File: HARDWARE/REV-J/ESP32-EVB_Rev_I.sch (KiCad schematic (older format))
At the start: 151 parts, among them CON1 TB3 DG306-5.0-3P, CON2 TB3 DG306-5.0-3P, Q1 BC817-40(SOT23), Q2 BC817-40(SOT23), Q3 Q12MHz/20pF/30ppm/2P/HC-49SM(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, Q4 BC817-40(SOT23), Q5 BC817-40(SOT23), Q7 BC817-40(SOT23), U1 BL4054B-42TPRN(SOT23-5), U10 BAT54C(SOT23-3), U2 SY8089AAAC(SOT23-5), U3 ESP-WROOM-32, U4 LAN8710A-EZC(QFN32), U5 CH340T(SSOP20W), U6 MCP2562-E/SN(SOIC-8_150mil), U7 RPM7236-H8, U8 NCP303LSN27T1G(SOT-23-5), U9 BAT54C(SOT23-3)

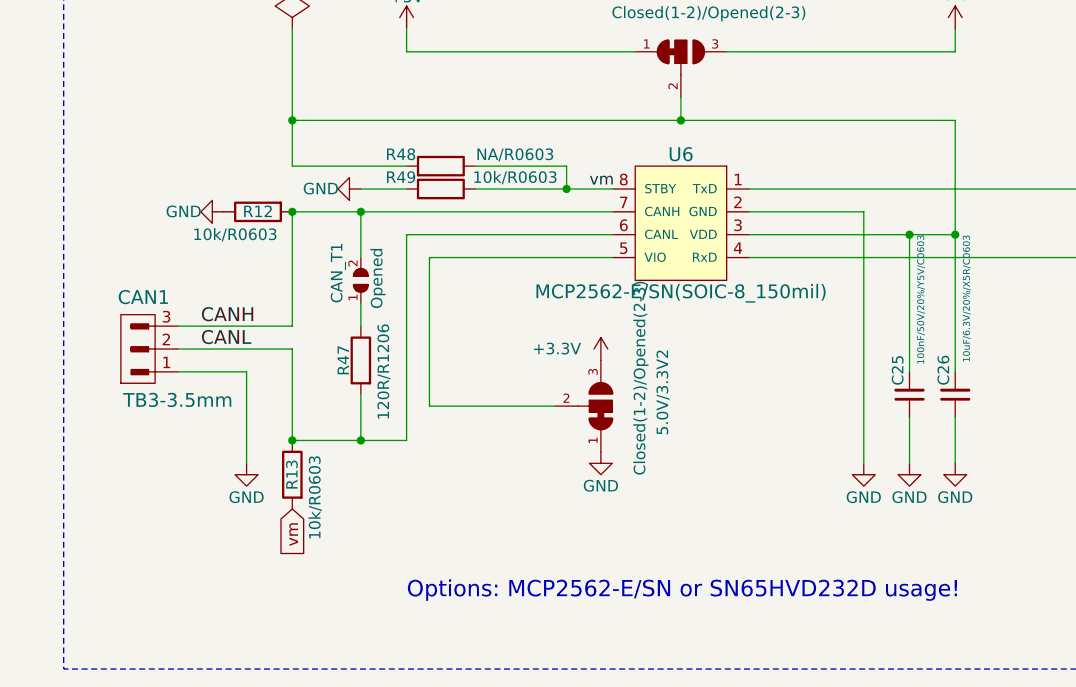
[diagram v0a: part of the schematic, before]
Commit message: Update 434121043836 (rev1).stp, 5040771891.stp, and 173 more files...
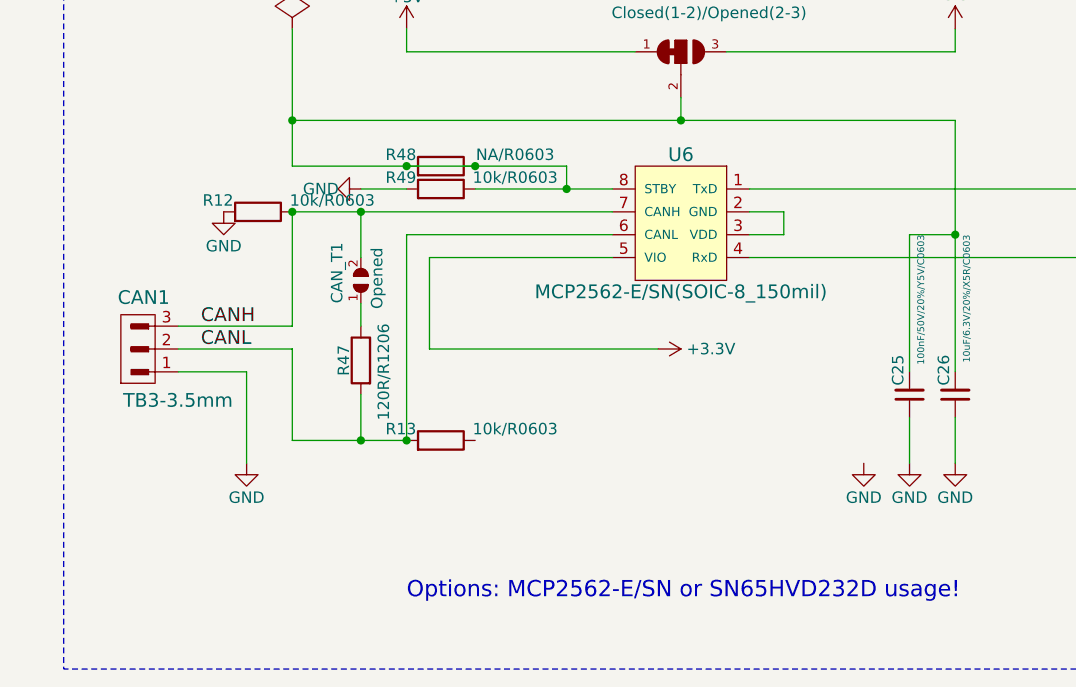
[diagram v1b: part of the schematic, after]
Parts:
- removed 5.0V/3.3V2: Closed(1-2)/Opened(2-3), OLIMEX_Jumpers-FP:SJ_2_SMALL_12_TIED, symbol ESP32-EVB_Rev_I:SJ2W_Closed(1-2)
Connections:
- net labels removed: vm
- wire segments 689 -> 690
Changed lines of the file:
@@
 	13900 13400 13900 13900
 Connection ~ 13900 13900
-Connection ~ 13700 13900
-Wire Wire Line
-	13000 13900 13700 13900
 Wire Wire Line
 	15600 13700 13000 13700
@@
 	13000 14000 15600 14000
 Wire Wire Line
-	13000 13800 13500 13800
-Wire Wire Line
-	13500 13800 13500 14900
+	13000 13800 13150 13800
 Wire Wire Line
 	19900 7800 18800 7800
@@
 	12400 14000 11600 14000
 Wire Wire Line
+	11600 14000 11600 14400
+Wire Wire Line
+	11600 14400 12600 14400
+Wire Wire Line
 	2900 1800 2900 2100
 Wire Wire Line
@@
 Wire Wire Line
 	13700 13900 13700 14500
+$Comp
+L ESP32-EVB_Rev_I:+3.3V #PWR0101
+U 1 1 5B27C8D3
+P 12600 14400
+F 0 "#PWR0101" H 12600 14250 50  0001 C CNN
+F 1 "+3.3V" V 12600 14525 50  0000 L CNN
+F 2 "" H 12600 14400 60  0000 C CNN
+F 3 "" H 12600 14400 60  0000 C CNN
+	1    12600 14400
+	0    1    1    0
+$EndComp
 $Comp
 L ESP32-EVB_Rev_I:MCP2562-E_SN(SOIC-8_150mil) U6
@@
 	-1   0    0    1
 $EndComp
-$Comp
-L ESP32-EVB_Rev_I:SJ2W_Closed(1-2) 5.0V/3.3V2
-U 1 1 6188D1A4
-P 12350 14650
-F 0 "5.0V/3.3V2" V 12650 14400 50  0000 L BNN
-F 1 "Closed(1-2)/Opened(2-3)" V 12550 14100 50  0000 L BNN
-F 2 "OLIMEX_Jumpers-FP:SJ_2_SMALL_12_TIED" H 12380 14800 20  0001 C CNN
-F 3 "" H 12350 14650 60  0000 C CNN
-	1    12350 14650
-	1    0    0    1
-$EndComp
-$Comp
-L ESP32-EVB_Rev_I:+3.3V #PWR0101
-U 1 1 5B27C8D3
-P 12350 14450
-F 0 "#PWR0101" H 12350 14300 50  0001 C CNN
-F 1 "+3.3V" H 12050 14500 50  0000 L CNN
-F 2 "" H 12350 14450 60  0000 C CNN
-F 3 "" H 12350 14450 60  0000 C CNN
-	1    12350 14450
-	1    0    0    -1
-$EndComp
-Wire Wire Line
-	12150 14650 11600 14650
-Wire Wire Line
-	11600 14000 11600 14650
-$Comp
-L ESP32-EVB_Rev_I:GND #PWR0114
-U 1 1 61ADEB7D
-P 12350 14850
-F 0 "#PWR0114" H 12350 14600 50  0001 C CNN
-F 1 "GND" H 12350 14700 50  0000 C CNN
-F 2 "" H 12350 14850 60  0000 C CNN
-F 3 "" H 12350 14850 60  0000 C CNN
-	1    12350 14850
-	1    0    0    -1
-$EndComp
-Connection ~ 11000 13800
+Wire Wire Line
+	13000 13900 13150 13900
+Wire Wire Line
+	13150 13800 13150 13900
+Wire Wire Line
+	11500 13600 11800 13600
+Connection ~ 11500 13600
+Connection ~ 11800 13600
 $Comp
 L ESP32-EVB_Rev_I:R R12
-U 1 1 61AF20A4
+U 1 1 61A8BD6D
 P 10850 13800
-F 0 "R12" H 10850 13800 50  0000 C CNN
-F 1 "10k/R0603" H 10750 13900 50  0000 C CNN
+F 0 "R12" H 11025 13850 50  0000 C CNN
+F 1 "10k/R0603" H 10525 13850 50  0000 C CNN
 F 2 "OLIMEX_RLC-FP:R_0603_5MIL_DWS" V 10780 13800 30  0001 C CNN
 F 3 "" H 10850 13800 30  0000 C CNN
 	1    10850 13800
-	1    0    0    1
-$EndComp
+	-1   0    0    -1
+$EndComp
+Connection ~ 11000 13800
 $Comp
 L ESP32-EVB_Rev_I:R R13
-U 1 1 61B8557C
-P 11000 14950
-F 0 "R13" H 11000 14950 50  0000 C CNN
-F 1 "10k/R0603" H 11100 14850 50  0000 C CNN
-F 2 "OLIMEX_RLC-FP:R_0603_5MIL_DWS" V 10930 14950 30  0001 C CNN
-F 3 "" H 11000 14950 30  0000 C CNN
-	1    11000 14950
-	0    -1   1    0
-$EndComp
-Connection ~ 11000 14800
-$Comp
-L ESP32-EVB_Rev_I:GND #PWR0115
-U 1 1 61B984EC
+U 1 1 61A8C506
+P 11650 14800
+F 0 "R13" H 11825 14850 50  0000 C CNN
+F 1 "10k/R0603" H 11325 14850 50  0000 C CNN
+F 2 "OLIMEX_RLC-FP:R_0603_5MIL_DWS" V 11580 14800 30  0001 C CNN
+F 3 "" H 11650 14800 30  0000 C CNN
+	1    11650 14800
+	-1   0    0    -1
+$EndComp
+Connection ~ 11500 14800
+$Comp
+L ESP32-EVB_Rev_I:GND #PWR0114
+U 1 1 61A8D549
 P 10700 13800
-F 0 "#PWR0115" H 10700 13550 50  0001 C CNN
-F 1 "GND" V 10700 13625 50  0000 C CNN
+F 0 "#PWR0114" H 10700 13550 50  0001 C CNN
+F 1 "GND" H 10700 13650 50  0000 C CNN
 F 2 "" H 10700 13800 60  0000 C CNN
 F 3 "" H 10700 13800 60  0000 C CNN
 	1    10700 13800
-	0    1    -1   0
-$EndComp
-Text GLabel 11000 15100 3    50   Input ~ 0
-vm
-Text Label 12300 13700 0    50   ~ 0
-vm
+	1    0    0    -1
+$EndComp
 $EndSCHEMATC
